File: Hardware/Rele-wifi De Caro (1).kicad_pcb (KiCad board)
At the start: 2 copper layers, 78.3 x 71.2 mm, 38 parts, among them IC1 MC7805CD2TG, J1 Screw_Terminal_01x03, J2 Screw_Terminal_01x03, J3 Screw_Terminal_01x03, J4 Screw_Terminal_01x03, J5 Screw_Terminal_01x02, K1 PR13-5V-450-1C, K2 PR13-5V-450-1C, K3 PR13-5V-450-1C, K4 PR13-5V-450-1C, Q1 PC817-B, Q2 PC817-B, Q3 BC547, Q4 BC547, Q5 PC817-B, Q6 BC547, Q7 PC817-B, Q8 BC547, SW1 SW_DPST_x2, U2 ESP32-CAM

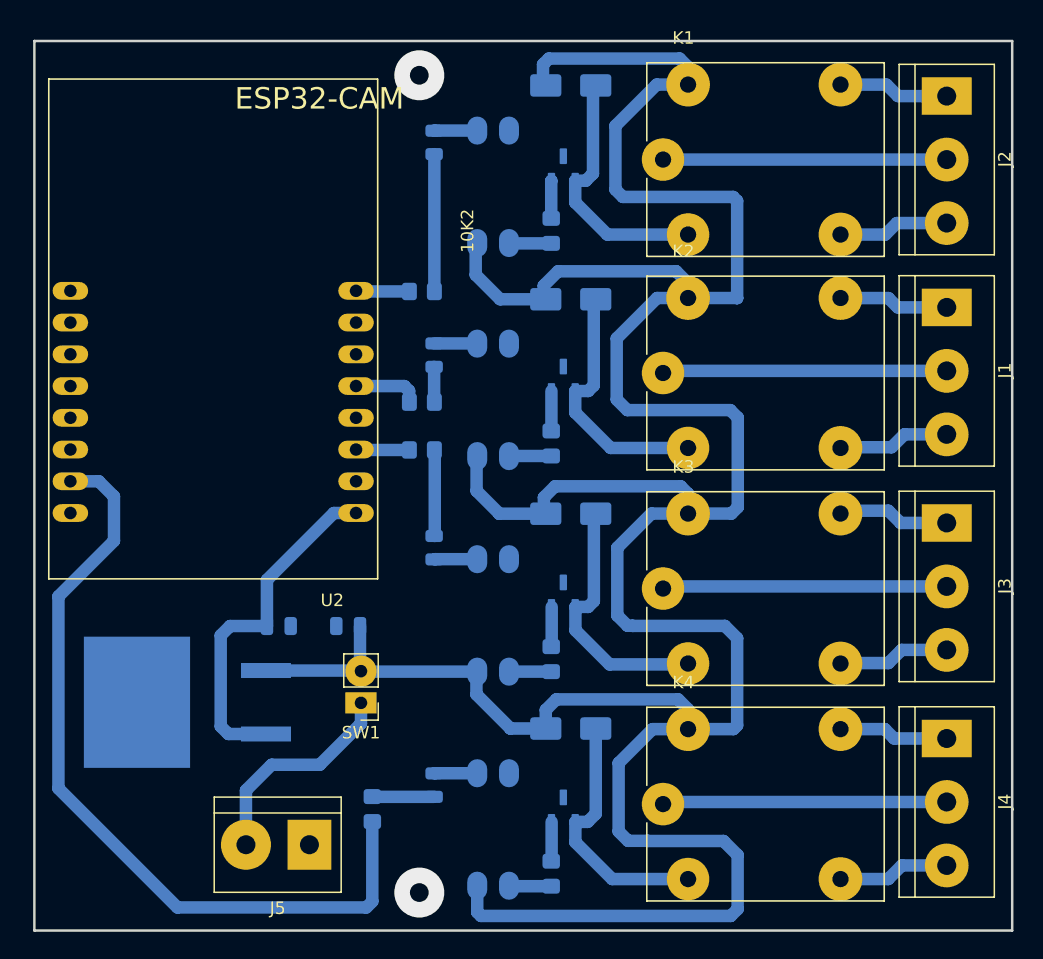
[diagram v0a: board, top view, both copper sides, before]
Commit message: PCB terminado 2.0
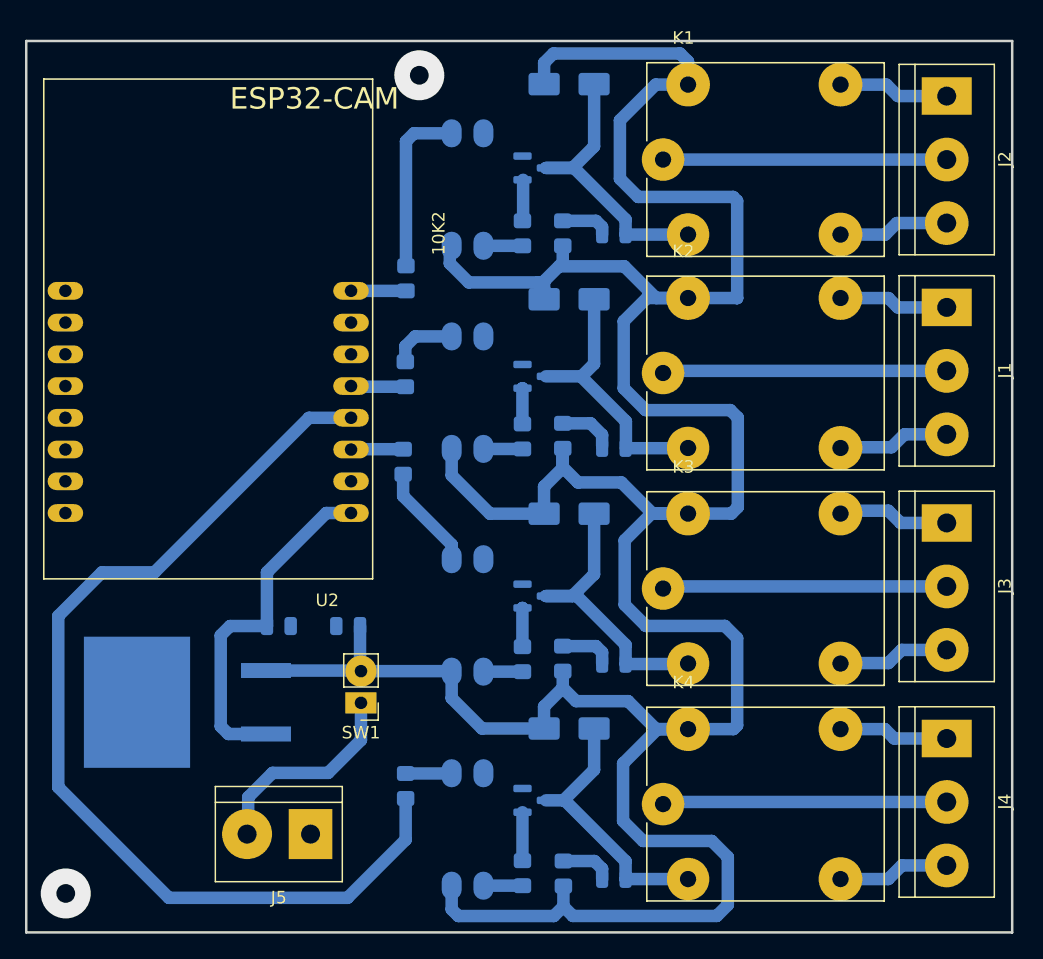
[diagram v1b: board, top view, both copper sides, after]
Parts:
- removed Q3, Q4, Q6, Q8: BC547, bc547 smd:SOT95P230X110-3N
- added Q10: BC847, Package_TO_SOT_SMD:SOT-23, B.Cu at (167.5, 104.0)
- added Q11: BC847, Package_TO_SOT_SMD:SOT-23, B.Cu at (167.5, 53.3)
- added Q12: BC847, Package_TO_SOT_SMD:SOT-23, B.Cu at (167.5, 70.0)
- added Q9: BC847, Package_TO_SOT_SMD:SOT-23, B.Cu at (167.5, 87.6)
- added R5: 680, Resistor_SMD:R_0805_2012Metric_Pad1.20x1.40mm_HandSolder, B.Cu at (169.8, 58.6)
- added R6: 680, Resistor_SMD:R_0805_2012Metric_Pad1.20x1.40mm_HandSolder, B.Cu at (169.8, 74.8)
- added R7: 680, Resistor_SMD:R_0805_2012Metric_Pad1.20x1.40mm_HandSolder, B.Cu at (169.8, 92.6)
- added R8: 680, Resistor_SMD:R_0805_2012Metric_Pad1.20x1.40mm_HandSolder, B.Cu at (169.8, 109.8)
- moved D5 17.1 mm to (173.9, 93.0), turned to 180 degrees
- moved D7 16.2 mm to (173.9, 110.3), turned to 180 degrees
- moved D1 16.2 mm to (173.9, 75.8), turned to 180 degrees
- moved D2 16.2 mm to (173.9, 58.7), turned to 180 degrees
- moved R4 3.24 mm to (157.2, 102.8)
- moved R1 2.59 mm to (157.2, 69.8), turned to 90 degrees
- moved 10K1 2.37 mm to (166.5, 74.8)
- moved 10K2 2.31 mm to (166.5, 58.6)
- moved 10K4 2.30 mm to (166.5, 109.8)
- moved 10K3 2.30 mm to (166.5, 92.7)
- moved Q1 2.13 mm to (162.2, 71.3)
- moved Q2 2.06 mm to (162.2, 55.1)
- moved Q5 2.05 mm to (162.2, 89.2)
- moved Q7 2.05 mm to (162.2, 106.3)
- moved R3 1.77 mm to (157.0, 76.8), turned to -90 degrees
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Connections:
- D3 pad 2: Net-(D3-A) -> Net-(D2-K)
- D4 pad 2: Net-(D4-A) -> Net-(D1-K)
- D6 pad 2: Net-(D6-A) -> Net-(D5-K)
- D8 pad 2: Net-(D8-A) -> Net-(D7-K)
- K1 pad A2: Net-(D3-A) -> Net-(D2-K)
- K2 pad A2: Net-(D4-A) -> Net-(D1-K)
- K3 pad A2: Net-(D6-A) -> Net-(D5-K)
- K4 pad A2: Net-(D8-A) -> Net-(D7-K)
- Q1 pad 1: Net-(D1-K) -> Net-(Q1-Pad1)
- Q2 pad 1: Net-(D2-K) -> Net-(Q2-Pad1)
- Q5 pad 1: Net-(D5-K) -> Net-(Q5-Pad1)
- Q7 pad 1: Net-(D7-K) -> Net-(Q7-Pad1)
- R1 pad 2: Net-(D1-A) -> Net-(Q1-Pad1)
- R2 pad 2: Net-(D2-A) -> Net-(Q2-Pad1)
- R3 pad 2: Net-(D5-A) -> Net-(Q5-Pad1)
- R4 pad 1: GPIO 16 -> GPIO 13
- R4 pad 2: Net-(D7-A) -> Net-(Q7-Pad1)
- U2 pad P$15: GPIO 16 -> unconnected-(U2-IO16-PadP$15)
- U2 pad P$4: unconnected-(U2-IO13-PadP$4) -> GPIO 13
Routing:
- net GPIO 13: track 0.00 -> 80.4 mm
- net GPIO 16: track 64.9 -> 0.00 mm
- net Net-(D6-A): track 20.7 -> 0.00 mm
- net Net-(D5-K): track 3.34 -> 24.0 mm
- net Net-(D8-A): track 20.6 -> 0.00 mm
- net Net-(D3-A): track 20.5 -> 0.00 mm
- net Net-(D2-K): track 3.31 -> 23.8 mm
- net Net-(D4-A): track 20.5 -> 0.00 mm
- net Net-(D1-K): track 3.40 -> 21.6 mm
- net Net-(D7-K): track 3.42 -> 21.6 mm
- net Net-(Q2-Pad1): track 0.00 -> 13.7 mm
- net VCC: track 258.2 -> 267.4 mm
- net Net-(Q5-Pad1): track 0.00 -> 8.41 mm
- net Net-(D2-A): track 11.0 -> 3.86 mm
- net Net-(Q1-Pad1): track 0.00 -> 5.27 mm
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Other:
- board size 78.3 x 71.2 mm -> 78.9 x 71.3 mm
